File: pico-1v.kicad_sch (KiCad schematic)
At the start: 45 parts, among them J2 USB-C-2.0, J3 Header-1, J4 Header-2, J5 SWD, J6 USB_B_Micro, SW1 UK-B0273-SP25Y, SW2 USB Boot, SW4 SW_Slide_DPDT, U1 RP2040, U2 NCP1117-1.8_SOT223, U3 NCP1117-3.3_SOT223, U4 AT25FF161A-SSHN-T, Y1 ECS-3225MV-120-BN-TR3

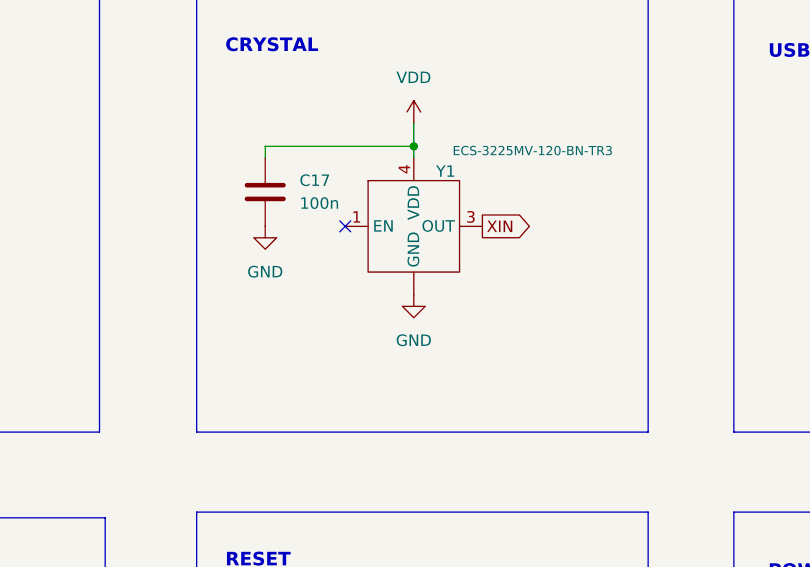
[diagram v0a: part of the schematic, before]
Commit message: Updated some stuff
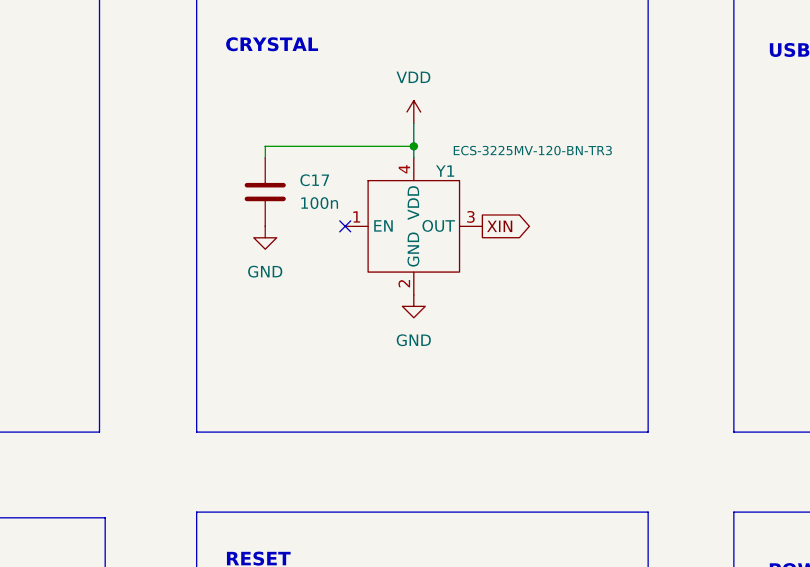
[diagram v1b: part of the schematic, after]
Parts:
- Y1: footprint (none) -> Oscillator:Oscillator_SMD_Abracon_ASE-4Pin_3.2x2.5mm
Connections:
- net GND: now also Y1.2 (GND); no longer Y1. (GND)
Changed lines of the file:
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@@
 			)
 		)
-		(property "Footprint" ""
+		(property "Footprint" "Oscillator:Oscillator_SMD_Abracon_ASE-4Pin_3.2x2.5mm"
 			(at 104.14 187.96 0)
 			(effects
@@
 		(pin "1"
 		)
-		(pin ""
+		(pin "2"
 		)
 		(pin "4"

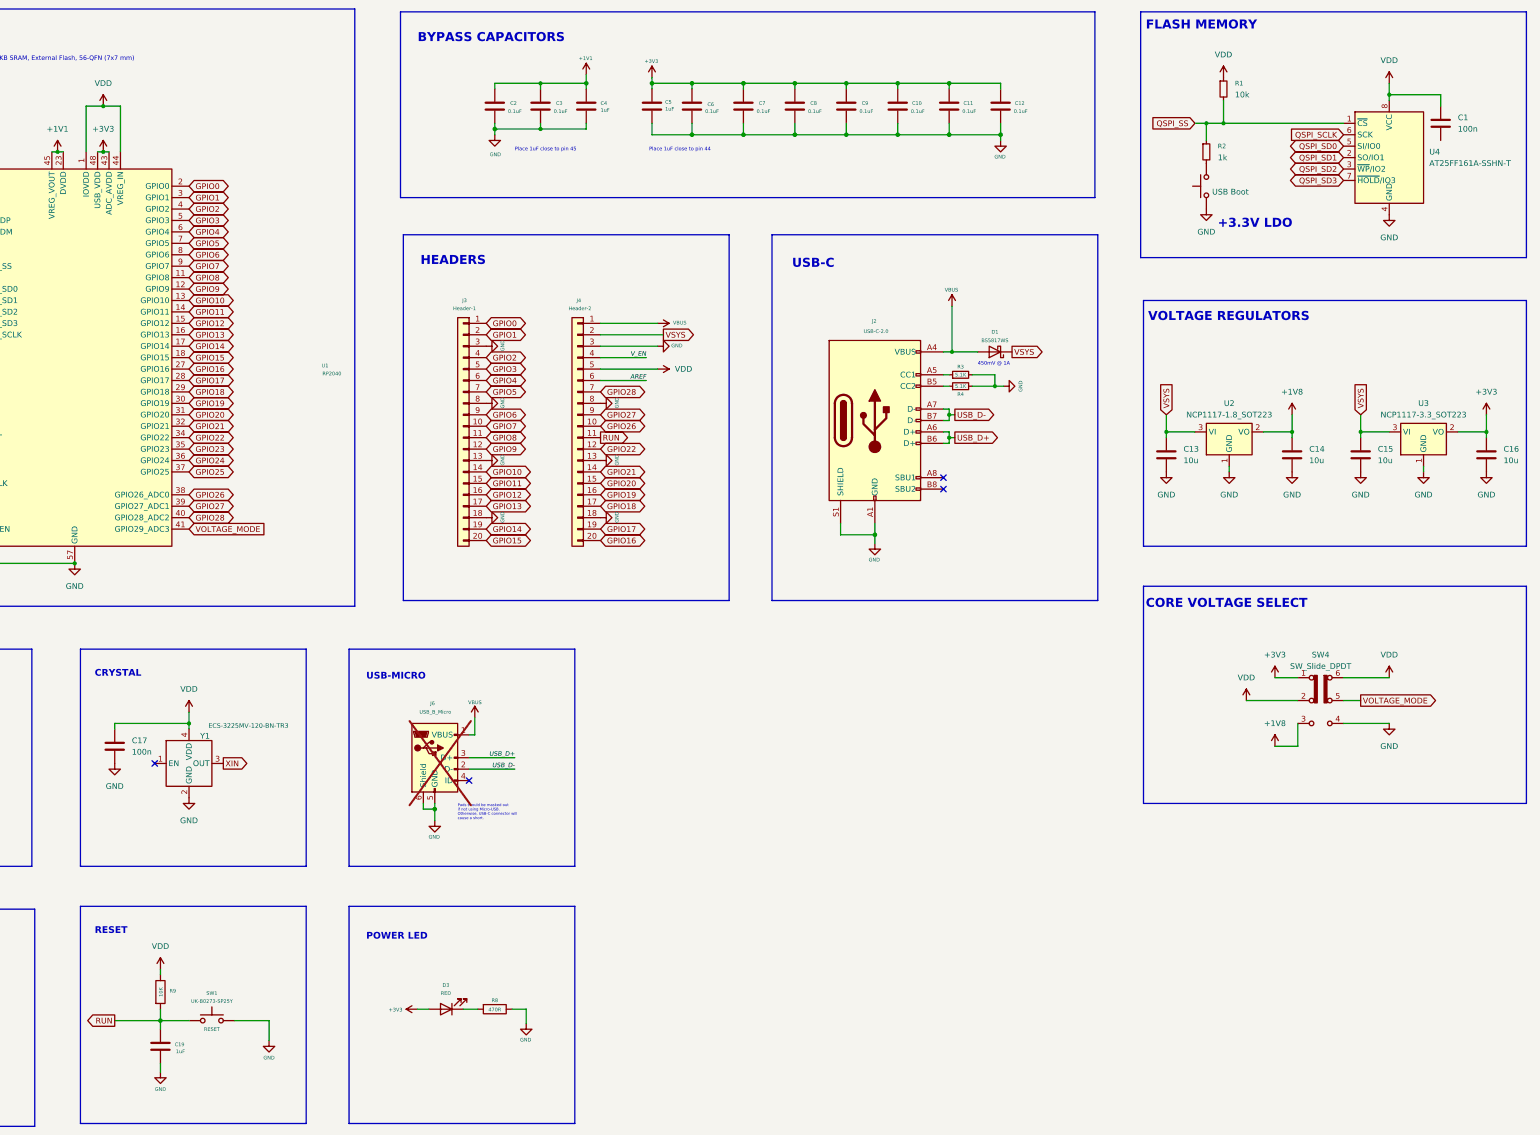
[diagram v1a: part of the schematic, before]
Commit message: PCB
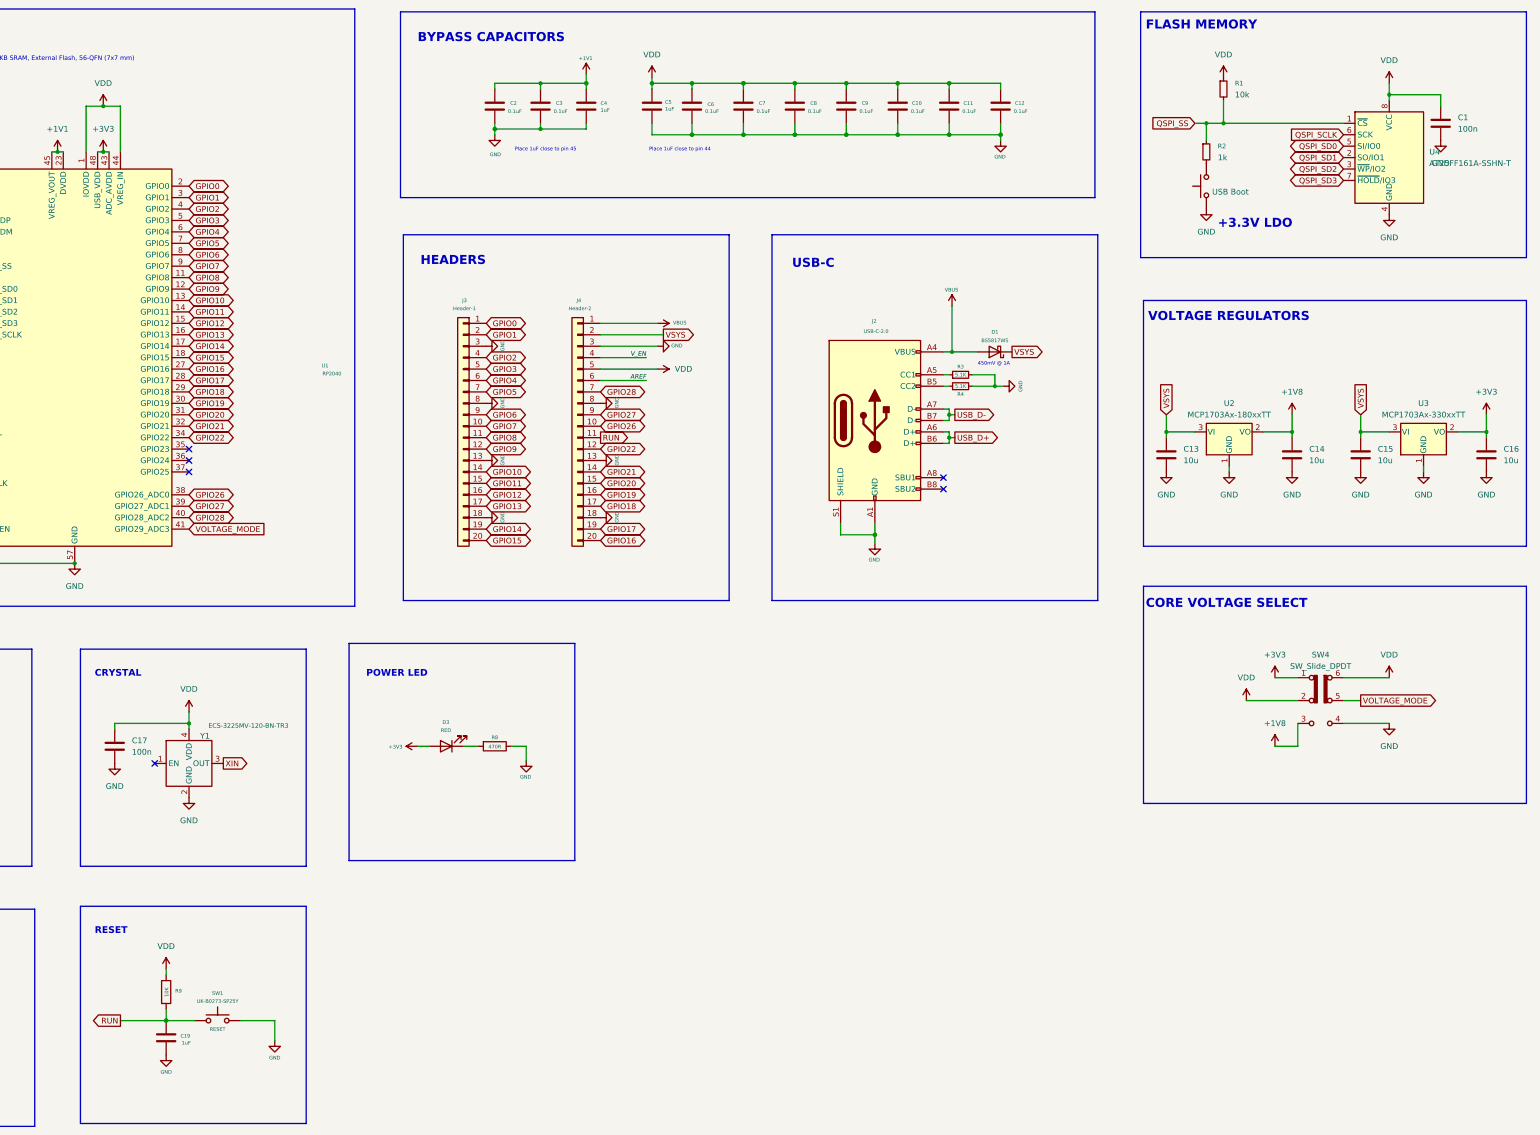
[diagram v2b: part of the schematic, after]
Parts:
- removed J6: USB_B_Micro, Connector_USB:USB_Micro-B_Molex-105017-0001, symbol Connector:USB_B_Micro
- removed U2: NCP1117-1.8_SOT223, Package_TO_SOT_SMD:SOT-223-3_TabPin2, symbol Regulator_Linear:NCP1117-1.8_SOT223
- removed U3: NCP1117-3.3_SOT223, Package_TO_SOT_SMD:SOT-223-3_TabPin2, symbol Regulator_Linear:NCP1117-3.3_SOT223
- added U2: MCP1703Ax-180xxTT, Package_TO_SOT_SMD:SOT-23, symbol Regulator_Linear:MCP1703Ax-180xxTT
- added U3: MCP1703Ax-330xxTT, Package_TO_SOT_SMD:SOT-23, symbol Regulator_Linear:MCP1703Ax-330xxTT
- Y1: footprint Oscillator:Oscillator_SMD_Abracon_ASE-4Pin_3.2x2.5mm -> ExtraFootprints:ECS-3225MV-120-BN-TR3
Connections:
- net +1V8: now also U2.2 (VO)
- net +3V3: now also U3.2 (VO); no longer C10.1, C11.1, C12.1, C5.1, C6.1, C7.1, C8.1, C9.1
- net GND: now also C1.2, U2.1 (GND), U3.1 (GND)
- net VDD: now also C10.1, C11.1, C12.1, C5.1, C6.1, C7.1, C8.1, C9.1
- net VSYS: now also U2.3 (VI), U3.3 (VI)
- net GPIO23: no longer names the net of U1.35 (GPIO23)
- net GPIO24: no longer names the net of U1.36 (GPIO24)
- net GPIO25: no longer names the net of U1.37 (GPIO25)
- no-connect marks 5 -> 7
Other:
- note removed: "Pads should be masked out if not using Micro-USB. Otherwise, USB-C connector will cause a short."
- note removed: "USB-MICRO"
- moved on the sheet: C19, D3, R8, R9, SW1
